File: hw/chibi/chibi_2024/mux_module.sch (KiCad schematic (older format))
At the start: 7 parts, among them U9 MBI5026

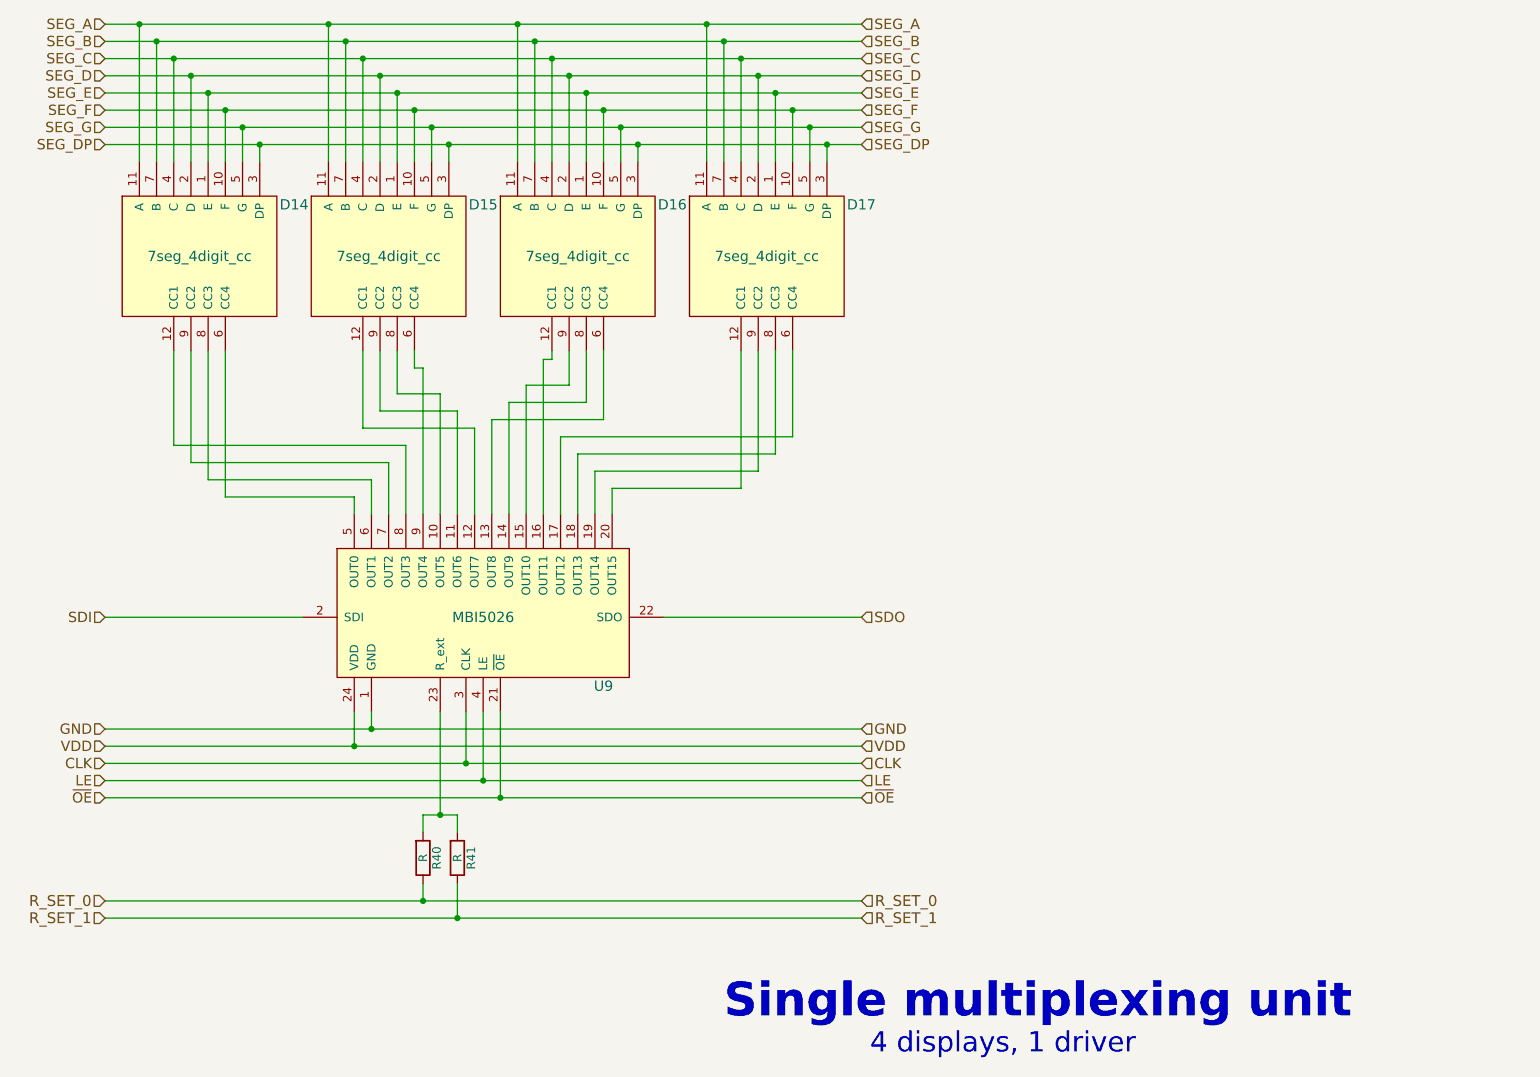
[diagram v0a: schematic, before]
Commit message: Foo
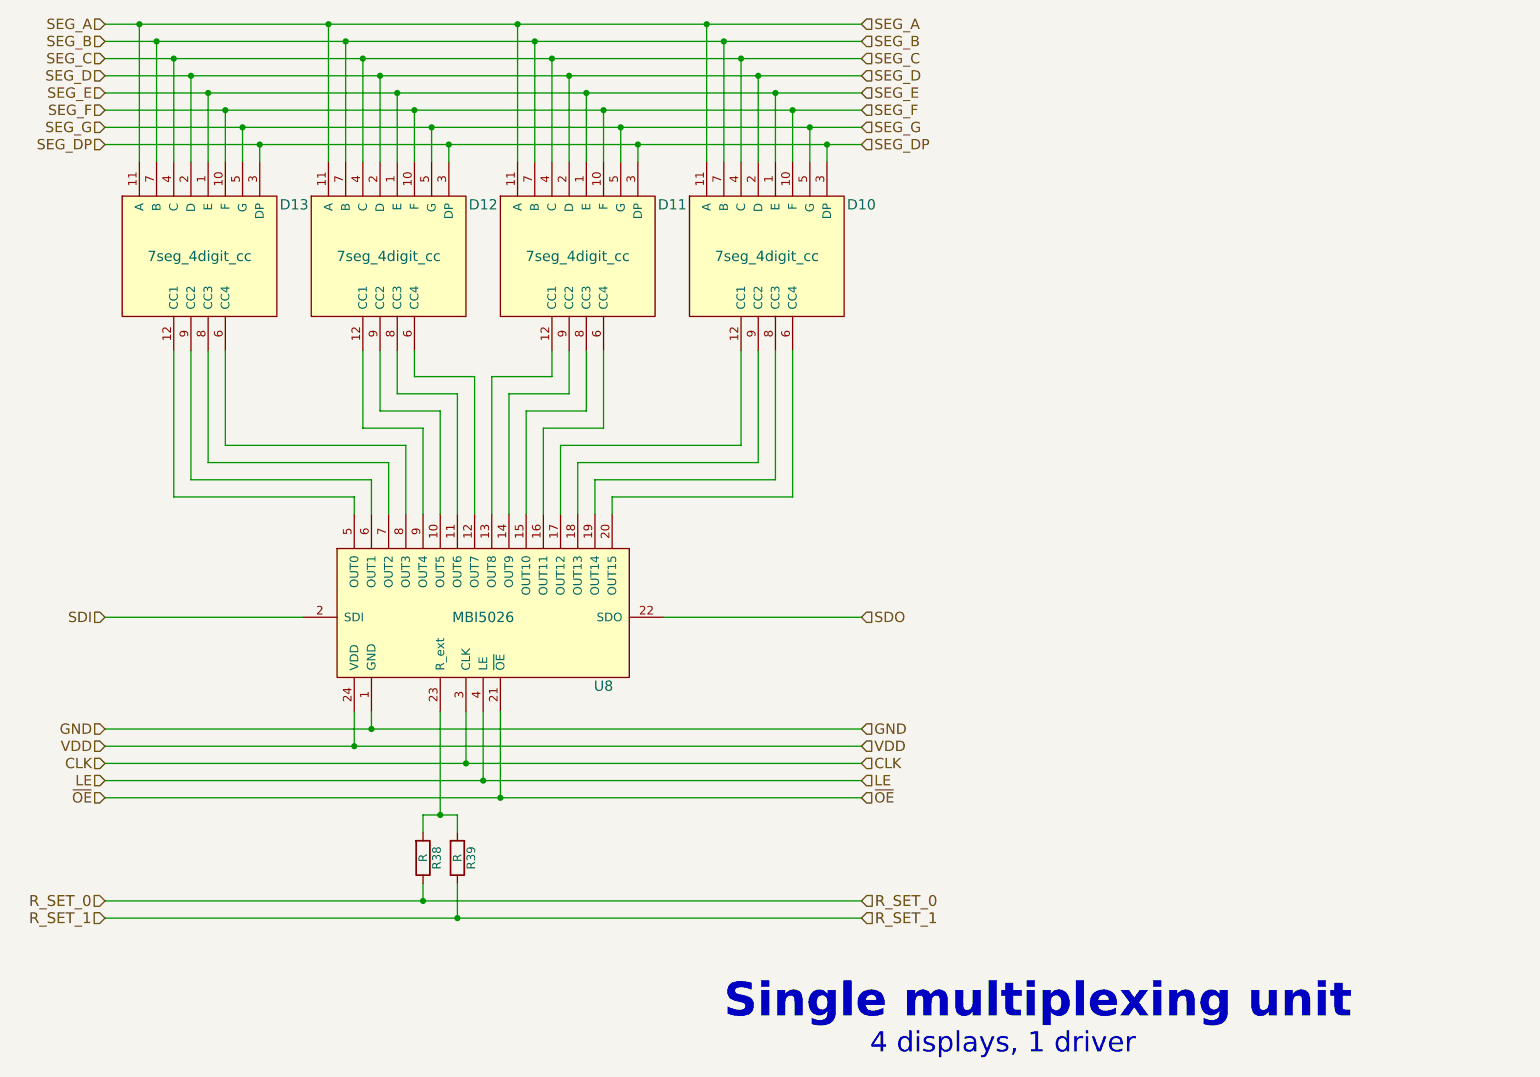
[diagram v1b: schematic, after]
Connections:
- net at D14.12 (CC1): now also U9.17 (OUT12); no longer U9.8 (OUT3)
- net at D14.6 (CC4): now also U9.20 (OUT15); no longer U9.5 (OUT0)
- net at D14.8 (CC3): now also U9.19 (OUT14); no longer U9.6 (OUT1)
- net at D14.9 (CC2): now also U9.18 (OUT13); no longer U9.7 (OUT2)
- net at D15.12 (CC1): now also U9.13 (OUT8); no longer U9.12 (OUT7)
- net at D15.6 (CC4): now also U9.16 (OUT11); no longer U9.9 (OUT4)
- net at D15.8 (CC3): now also U9.15 (OUT10); no longer U9.10 (OUT5)
- net at D15.9 (CC2): now also U9.14 (OUT9); no longer U9.11 (OUT6)
- net at D16.12 (CC1): now also U9.9 (OUT4); no longer U9.16 (OUT11)
- net at D16.6 (CC4): now also U9.12 (OUT7); no longer U9.13 (OUT8)
- net at D16.8 (CC3): now also U9.11 (OUT6); no longer U9.14 (OUT9)
- net at D16.9 (CC2): now also U9.10 (OUT5); no longer U9.15 (OUT10)
- net at D17.12 (CC1): now also U9.5 (OUT0); no longer U9.20 (OUT15)
- net at D17.6 (CC4): now also U9.8 (OUT3); no longer U9.17 (OUT12)
- net at D17.8 (CC3): now also U9.7 (OUT2); no longer U9.18 (OUT13)
- net at D17.9 (CC2): now also U9.6 (OUT1); no longer U9.19 (OUT14)
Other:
- moved on the sheet: D10, D11, D12, D13
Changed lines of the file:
@@
 L 7seg_4digit_cc D14
 U 1 1 5900990E
-P 4250 2450
+P 7550 2450
 AR Path="/5901390A/5900990E" Ref="D14"  Part="1"
 AR Path="/59008B1D/5900990E" Ref="D10"  Part="1"
-F 0 "D14" H 4800 2750 60  0000 C CNN
+F 0 "D10" H 8100 2750 60  0000 C CNN
+F 1 "7seg_4digit_cc" H 7550 2450 60  0000 C CNN
+F 2 "Displays_7-Segment:Cx56-12" H 8550 2350 60  0001 C CNN
+F 3 "" H 8550 2350 60  0001 C CNN
+	1    7550 2450
+	1    0    0    -1
+$EndComp
+$Comp
+L 7seg_4digit_cc D15
+U 1 1 59009915
+P 6450 2450
+AR Path="/5901390A/59009915" Ref="D15"  Part="1"
+AR Path="/59008B1D/59009915" Ref="D11"  Part="1"
+F 0 "D11" H 7000 2750 60  0000 C CNN
+F 1 "7seg_4digit_cc" H 6450 2450 60  0000 C CNN
+F 2 "Displays_7-Segment:Cx56-12" H 7450 2350 60  0001 C CNN
+F 3 "" H 7450 2350 60  0001 C CNN
+	1    6450 2450
+	1    0    0    -1
+$EndComp
+$Comp
+L 7seg_4digit_cc D16
+U 1 1 5900991C
+P 5350 2450
+AR Path="/5901390A/5900991C" Ref="D16"  Part="1"
+AR Path="/59008B1D/5900991C" Ref="D12"  Part="1"
+F 0 "D12" H 5900 2750 60  0000 C CNN
+F 1 "7seg_4digit_cc" H 5350 2450 60  0000 C CNN
+F 2 "Displays_7-Segment:Cx56-12" H 6350 2350 60  0001 C CNN
+F 3 "" H 6350 2350 60  0001 C CNN
+	1    5350 2450
+	1    0    0    -1
+$EndComp
+$Comp
+L 7seg_4digit_cc D17
+U 1 1 59009923
+P 4250 2450
+AR Path="/5901390A/59009923" Ref="D17"  Part="1"
+AR Path="/59008B1D/59009923" Ref="D13"  Part="1"
+F 0 "D13" H 4800 2750 60  0000 C CNN
 F 1 "7seg_4digit_cc" H 4250 2450 60  0000 C CNN
 F 2 "Displays_7-Segment:Cx56-12" H 5250 2350 60  0001 C CNN
@@
 $EndComp
 $Comp
-L 7seg_4digit_cc D15
-U 1 1 59009915
-P 5350 2450
-AR Path="/5901390A/59009915" Ref="D15"  Part="1"
-AR Path="/59008B1D/59009915" Ref="D11"  Part="1"
-F 0 "D15" H 5900 2750 60  0000 C CNN
-F 1 "7seg_4digit_cc" H 5350 2450 60  0000 C CNN
-F 2 "Displays_7-Segment:Cx56-12" H 6350 2350 60  0001 C CNN
-F 3 "" H 6350 2350 60  0001 C CNN
-	1    5350 2450
-	1    0    0    -1
-$EndComp
-$Comp
-L 7seg_4digit_cc D16
-U 1 1 5900991C
-P 6450 2450
-AR Path="/5901390A/5900991C" Ref="D16"  Part="1"
-AR Path="/59008B1D/5900991C" Ref="D12"  Part="1"
-F 0 "D16" H 7000 2750 60  0000 C CNN
-F 1 "7seg_4digit_cc" H 6450 2450 60  0000 C CNN
-F 2 "Displays_7-Segment:Cx56-12" H 7450 2350 60  0001 C CNN
-F 3 "" H 7450 2350 60  0001 C CNN
-	1    6450 2450
-	1    0    0    -1
-$EndComp
-$Comp
-L 7seg_4digit_cc D17
-U 1 1 59009923
-P 7550 2450
-AR Path="/5901390A/59009923" Ref="D17"  Part="1"
-AR Path="/59008B1D/59009923" Ref="D13"  Part="1"
-F 0 "D17" H 8100 2750 60  0000 C CNN
-F 1 "7seg_4digit_cc" H 7550 2450 60  0000 C CNN
-F 2 "Displays_7-Segment:Cx56-12" H 8550 2350 60  0001 C CNN
-F 3 "" H 8550 2350 60  0001 C CNN
-	1    7550 2450
-	1    0    0    -1
-$EndComp
-$Comp
 L MBI5026 U9
 U 1 1 5900992A
@@
 AR Path="/5901390A/5900992A" Ref="U9"  Part="1"
 AR Path="/59008B1D/5900992A" Ref="U8"  Part="1"
-F 0 "U9" H 6600 4950 60  0000 C CNN
+F 0 "U8" H 6600 4950 60  0000 C CNN
 F 1 "MBI5026" H 5900 4550 60  0000 C CNN
 F 2 "footprints:SSOP24-1.0" H 5900 4550 60  0001 C CNN
@@
 AR Path="/5901390A/590099AE" Ref="R41"  Part="1"
 AR Path="/59008B1D/590099AE" Ref="R39"  Part="1"
-F 0 "R41" V 5830 5950 50  0000 C CNN
+F 0 "R39" V 5830 5950 50  0000 C CNN
 F 1 "R" V 5750 5950 50  0000 C CNN
 F 2 "Resistors_SMD:R_0603_HandSoldering" V 5680 5950 50  0001 C CNN
@@
 AR Path="/59008B1D/590DC56C" Ref="R38"  Part="1"
 AR Path="/5901390A/590DC56C" Ref="R40"  Part="1"
-F 0 "R40" V 5630 5950 50  0000 C CNN
+F 0 "R38" V 5630 5950 50  0000 C CNN
 F 1 "R" V 5550 5950 50  0000 C CNN
 F 2 "Resistors_SMD:R_0603_HandSoldering" V 5480 5950 50  0001 C CNN
@@
 R_SET_0
 Wire Wire Line
-	4400 3000 4400 3850
-Wire Wire Line
-	4300 3000 4300 3750
-Wire Wire Line
 	3700 1800 8100 1800
 Wire Wire Line
@@
 Connection ~ 5750 6300
 Wire Wire Line
-	5150 3950 5150 3850
-Wire Wire Line
-	5150 3850 4400 3850
-Wire Wire Line
-	4300 3750 5250 3750
-Wire Wire Line
-	5250 3750 5250 3950
-Wire Wire Line
-	5350 3950 5350 3650
-Wire Wire Line
-	5350 3650 4200 3650
-Wire Wire Line
-	4100 3550 5450 3550
-Wire Wire Line
-	5450 3550 5450 3950
-Wire Wire Line
-	4200 3650 4200 3000
-Wire Wire Line
-	4100 3000 4100 3550
-Wire Wire Line
-	5500 3000 5500 3100
-Wire Wire Line
-	5500 3100 5550 3100
-Wire Wire Line
-	5550 3100 5550 3950
+	4100 3000 4100 3850
+Wire Wire Line
+	4100 3850 5150 3850
+Wire Wire Line
+	5150 3850 5150 3950
+Wire Wire Line
+	5250 3950 5250 3750
+Wire Wire Line
+	5250 3750 4200 3750
+Wire Wire Line
+	4200 3750 4200 3000
+Wire Wire Line
+	4300 3000 4300 3650
+Wire Wire Line
+	4300 3650 5350 3650
+Wire Wire Line
+	5350 3650 5350 3950
+Wire Wire Line
+	5450 3950 5450 3550
+Wire Wire Line
+	5450 3550 4400 3550
+Wire Wire Line
+	4400 3550 4400 3000
+Wire Wire Line
+	5200 3000 5200 3450
+Wire Wire Line
+	5200 3450 5550 3450
+Wire Wire Line
+	5550 3450 5550 3950
+Wire Wire Line
+	5650 3950 5650 3350
+Wire Wire Line
+	5650 3350 5300 3350
+Wire Wire Line
+	5300 3350 5300 3000
 Wire Wire Line
 	5400 3000 5400 3250
 Wire Wire Line
-	5400 3250 5650 3250
-Wire Wire Line
-	5650 3250 5650 3950
-Wire Wire Line
-	5300 3000 5300 3350
-Wire Wire Line
-	5300 3350 5750 3350
-Wire Wire Line
-	5750 3350 5750 3950
-Wire Wire Line
-	5200 3000 5200 3450
-Wire Wire Line
-	5200 3450 5850 3450
-Wire Wire Line
-	5850 3450 5850 3950
-Wire Wire Line
-	6300 3000 6300 3050
-Wire Wire Line
-	6300 3050 6250 3050
-Wire Wire Line
-	6250 3050 6250 3950
-Wire Wire Line
-	6400 3000 6400 3200
-Wire Wire Line
-	6400 3200 6150 3200
-Wire Wire Line
-	6150 3200 6150 3950
-Wire Wire Line
-	6050 3950 6050 3300
-Wire Wire Line
-	6050 3300 6500 3300
-Wire Wire Line
-	6500 3300 6500 3000
-Wire Wire Line
-	6600 3000 6600 3400
-Wire Wire Line
-	6600 3400 5950 3400
-Wire Wire Line
-	5950 3400 5950 3950
-Wire Wire Line
-	6350 3950 6350 3500
-Wire Wire Line
-	6350 3500 7700 3500
-Wire Wire Line
-	7700 3500 7700 3000
-Wire Wire Line
-	7600 3000 7600 3600
-Wire Wire Line
-	7600 3600 6450 3600
-Wire Wire Line
-	6450 3600 6450 3950
-Wire Wire Line
-	6550 3950 6550 3700
-Wire Wire Line
-	6550 3700 7500 3700
-Wire Wire Line
-	7500 3700 7500 3000
-Wire Wire Line
-	7400 3000 7400 3800
-Wire Wire Line
-	7400 3800 6650 3800
-Wire Wire Line
-	6650 3800 6650 3950
+	5400 3250 5750 3250
+Wire Wire Line
+	5750 3250 5750 3950
+Wire Wire Line
+	5850 3950 5850 3150
+Wire Wire Line
+	5850 3150 5500 3150
+Wire Wire Line
+	5500 3150 5500 3000
+Wire Wire Line
+	6300 3000 6300 3150
+Wire Wire Line
+	6300 3150 5950 3150
+Wire Wire Line
+	5950 3150 5950 3950
+Wire Wire Line
+	6050 3950 6050 3250
+Wire Wire Line
+	6050 3250 6400 3250
+Wire Wire Line
+	6400 3250 6400 3000
+Wire Wire Line
+	6500 3000 6500 3350
+Wire Wire Line
+	6500 3350 6150 3350
+Wire Wire Line
+	6150 3350 6150 3950
+Wire Wire Line
+	6250 3950 6250 3450
+Wire Wire Line
+	6250 3450 6600 3450
+Wire Wire Line
+	6600 3450 6600 3000
+Wire Wire Line
+	6350 3950 6350 3550
+Wire Wire Line
+	6350 3550 7400 3550
+Wire Wire Line
+	7400 3550 7400 3000
+Wire Wire Line
+	7500 3000 7500 3650
+Wire Wire Line
+	7500 3650 6450 3650
+Wire Wire Line
+	6450 3650 6450 3950
+Wire Wire Line
+	6550 3950 6550 3750
+Wire Wire Line
+	6550 3750 7600 3750
+Wire Wire Line
+	7600 3750 7600 3000
+Wire Wire Line
+	7700 3000 7700 3850
+Wire Wire Line
+	7700 3850 6650 3850
+Wire Wire Line
+	6650 3850 6650 3950
 $EndSCHEMATC
